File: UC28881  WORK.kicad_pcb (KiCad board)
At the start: 2 copper layers, 44.7 x 41.3 mm, 19 parts, among them J1 Screw_Terminal_01x03, U1 UCC28881

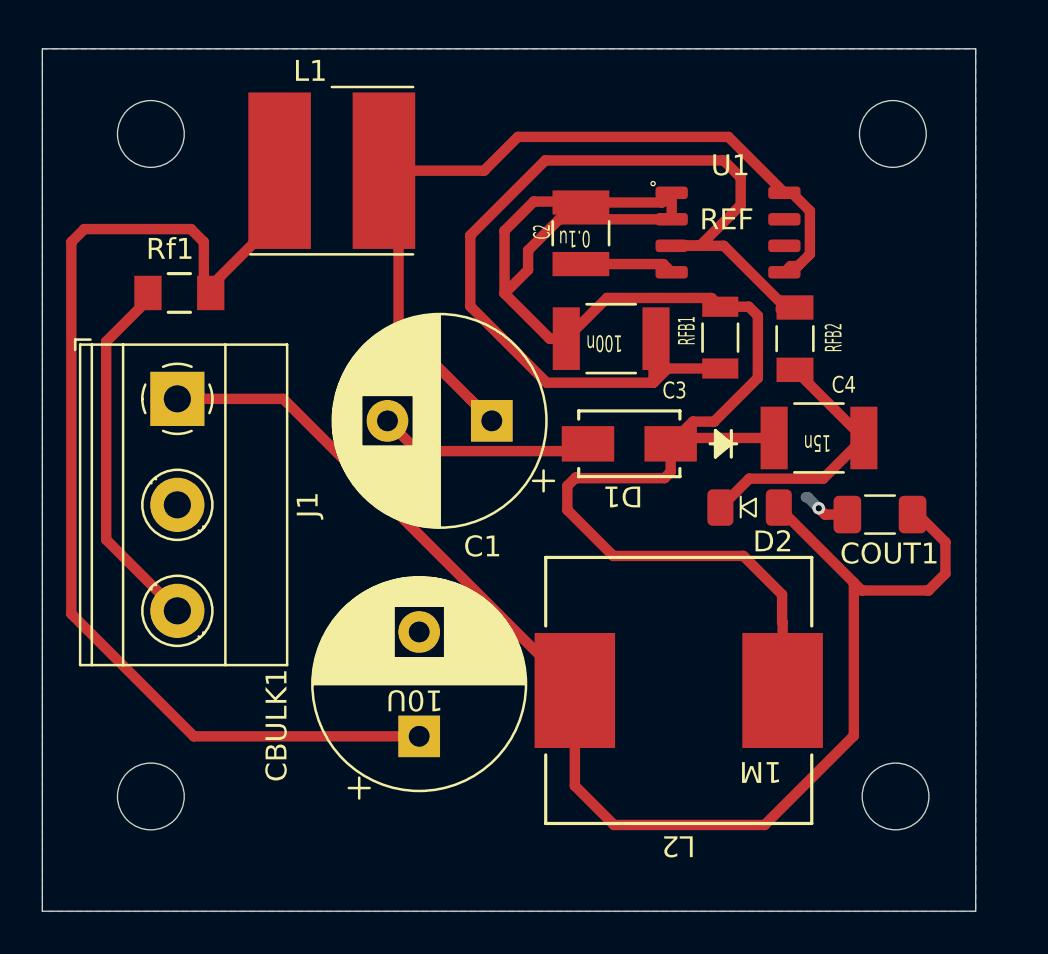
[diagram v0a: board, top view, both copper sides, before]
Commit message: edited pcb layout
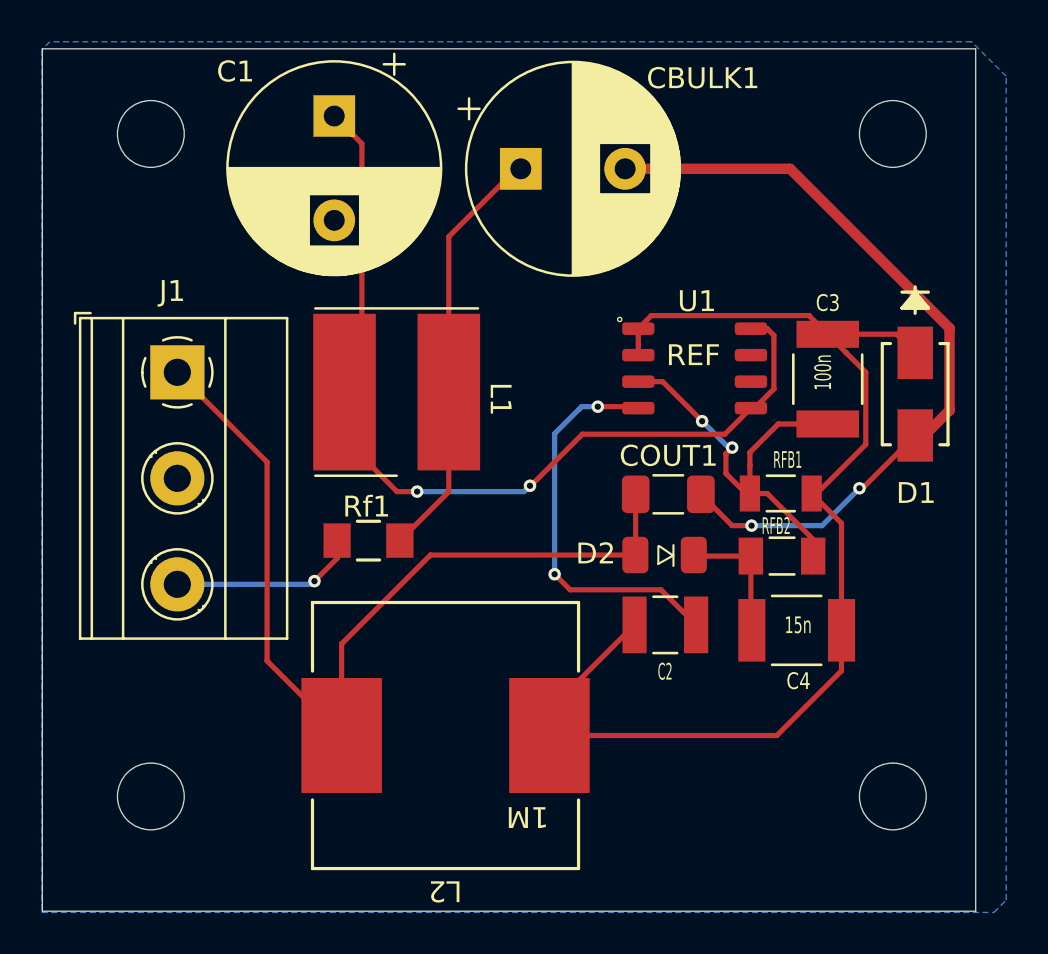
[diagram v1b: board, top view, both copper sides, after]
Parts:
- C2: value 0.1u -> (none)
- COUT1: value 47UF -> (none)
- D2: value M7 -> (none)
- RFB2: value 110k -> (none)
- U1: value UCC28881 -> (none)
- moved CBULK1 27.6 mm to (93.9, 39.8), turned to 0 degrees
- moved C2 19.2 mm to (100.9, 61.6), turned to 180 degrees
- moved C1 16.4 mm to (85.0, 37.2), turned to -90 degrees
- moved Rf1 14.9 mm to (86.6, 57.6)
- moved D1 13.9 mm to (112.8, 50.6), turned to -90 degrees
- moved L2 11.4 mm to (90.3, 66.9)
- moved L1 11.1 mm to (88.0, 50.5), turned to 180 degrees
- moved C3 10.6 mm to (108.6, 49.9), turned to 90 degrees
- moved RFB2 10.4 mm to (106.5, 58.3), turned to 180 degrees
- moved COUT1 10.2 mm to (101.0, 55.4), turned to 0 degrees
- moved C4 9.28 mm to (107.2, 61.9), turned to 0 degrees
- moved RFB1 8.01 mm to (106.4, 55.3), turned to 180 degrees
- moved U1 6.70 mm to (102.2, 49.3)
- moved D2 4.58 mm to (100.9, 58.4), turned to 180 degrees
- moved J1 1.27 mm to (77.5, 49.5)
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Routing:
- net Net-(CBULK1-Pad1): track 53.3 -> 20.3 mm
- net /Feedback pin: track 46.9 -> 19.8 mm, vias 0 -> 2
- net /GND: track 12.7 -> 37.5 mm, vias 1 -> 2
- net /10V_OUT_P: track 66.3 -> 43.8 mm
- net Net-(D1-K): track 75.1 -> 56.5 mm
- net Net-(U1-VDD): track 4.51 -> 19.1 mm, vias 0 -> 2
- net /HV_IN_P: track 17.6 -> 9.02 mm, vias 0 -> 1
- net Net-(D2-K): track 14.0 -> 6.33 mm
- net Net-(U1-DRAIN): track 42.4 -> 43.8 mm, vias 0 -> 2

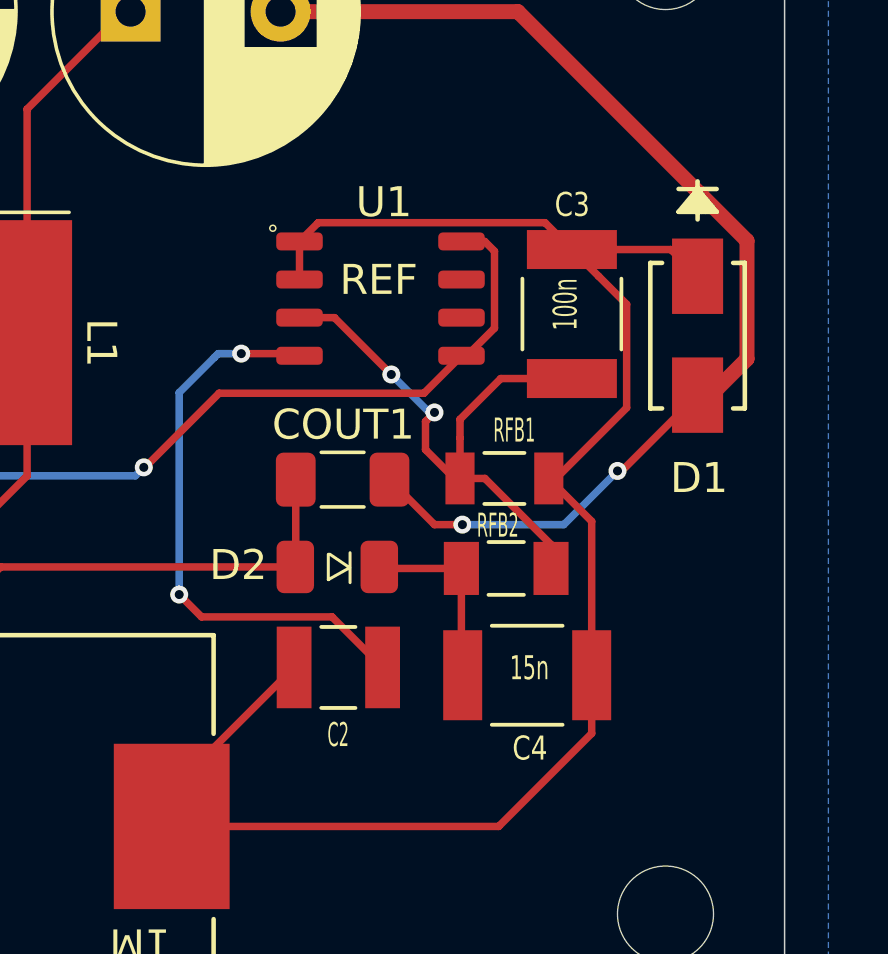
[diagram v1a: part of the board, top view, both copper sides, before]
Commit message: ADDED BOM
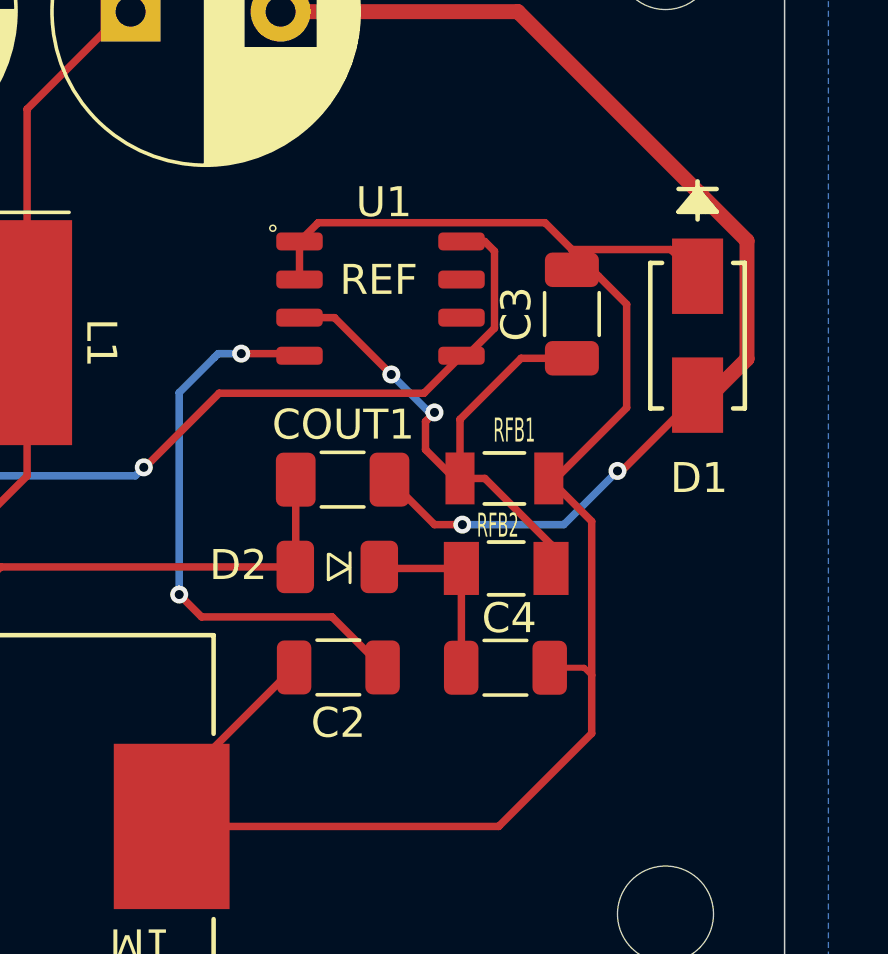
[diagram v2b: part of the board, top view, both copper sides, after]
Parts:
- C2: value (none) -> 0.1u; footprint C2:CAPC3225X88N -> Capacitor_SMD:C_1206_3216Metric
- C3: footprint C3:CAP_ECHU1H104GX9 -> Capacitor_SMD:C_1206_3216Metric
- C4: footprint C4:CAP_ECHU1H104GX9 -> Capacitor_SMD:C_1206_3216Metric
- COUT1: value (none) -> 47UF
- D2: value (none) -> M7
- RFB2: value (none) -> 110k
- U1: value (none) -> UCC28881
- moved C4 0.77 mm to (106.4, 61.6)
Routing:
- net Net-(D1-K): track 56.5 -> 58.0 mm
